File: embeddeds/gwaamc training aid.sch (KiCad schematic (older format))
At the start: 18 parts, among them J1 Conn_Coaxial, U1 LM334Z, U1-LSB MCP4162-502(0-5KΩ), U1-MSBs... MCP4162-104(0-100KΩ), U2 LM334Z, U2-LSB MCP4162-502(0-5KΩ), U2-MSBs... MCP4162-104(0-100KΩ), U3-A AD8244ARMZ, U3-B AD8244ARMZ, U3-C AD8244ARMZ, U3-D AD8244ARMZ, U4 74LV138

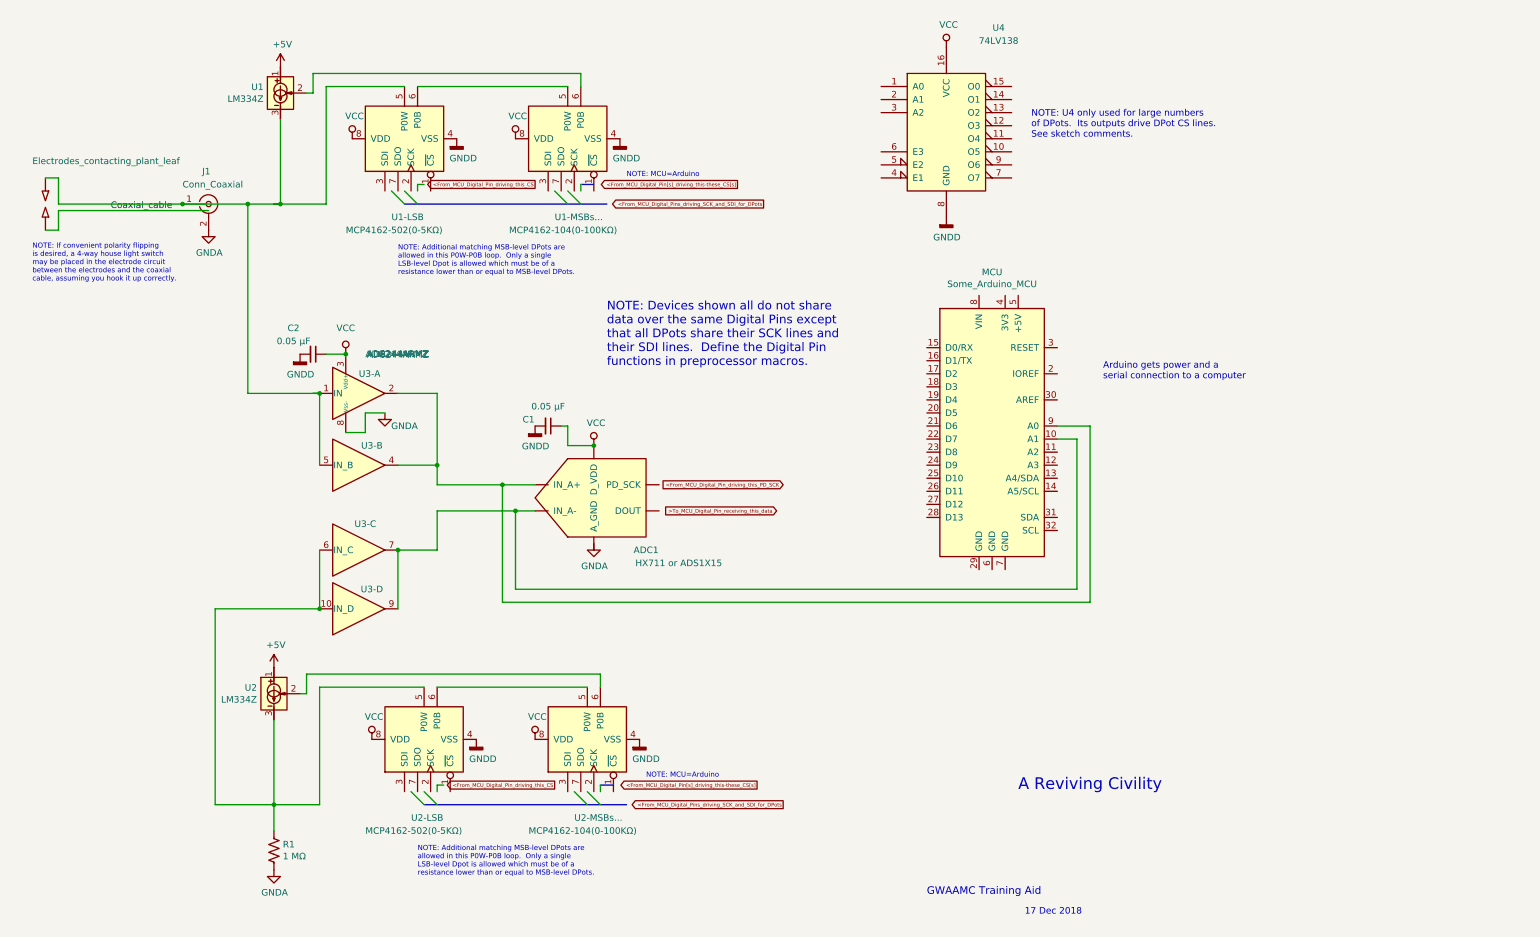
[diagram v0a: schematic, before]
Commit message: Schematic created in KiCad
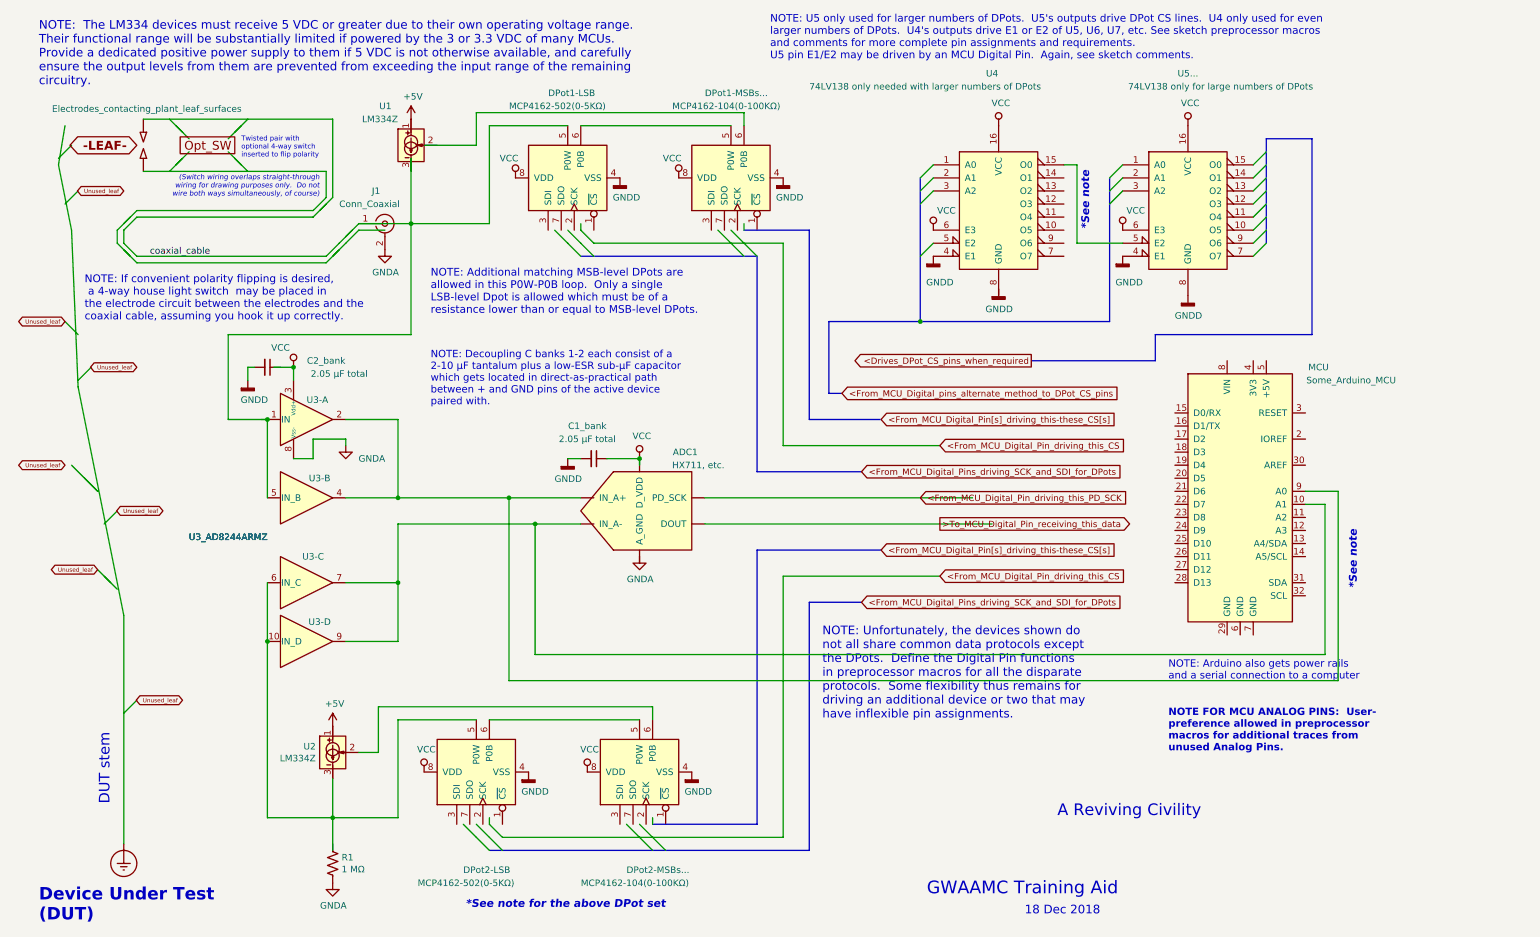
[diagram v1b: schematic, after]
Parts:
- added U4: 74LV138 only needed with larger numbers of DPots, symbol 74xx:74LS138
- ADC1: value HX711 or ADS1X15 -> HX711, etc.
- C1_bank: renamed from C1; value 0.05 µF -> 2.05 µF total
- C2_bank: renamed from C2; value 0.05 µF -> 2.05 µF total
- U3-A: value AD8244ARMZ -> (none)
- U3-B, U3-C, U3-D: value AD8244ARMZ -> U3_AD8244ARMZ
- U5...: renamed from U4; value 74LV138 -> 74LV138 only for large numbers of DPots
- renumbered U1-LSB to DPot1-LSB, U1-MSBs... to DPot1-MSBs..., U2-LSB to DPot2-LSB, U2-MSBs... to DPot2-MSBs..., Electrodes_contacting_plant_leaf to Electrodes_contacting_plant_leaf_surfaces
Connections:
- net labels added: -LEAF-, <Drives_DPot_CS_pins_when_required, <From_MCU_Digital_pins_alternate_method_to_DPot_CS_pins, Earth_Protective, Opt_SW, Unused_leaf, coaxial_cable
- net labels removed: Coaxial_cable
- wire segments 68 -> 90
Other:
- note added: "(Switch wiring overlaps straight-through \nwiring for drawing purposes only. Do not \nwire both ways simultaneously, of course)"
- note added: "*See note"
- note added: "*See note for the above DPot set"
- note added: "18 Dec 2018"
- note added: "DUT stem"
- note added: "Device Under Test \n(DUT)"
- note added: "NOTE FOR MCU ANALOG PINS: User-\npreference allowed in preprocessor \nmacros for additional traces from \nunused Analog Pins."
- note added: "NOTE: Arduino also gets power rails \nand a serial connection to a computer"
- note added: "NOTE: Decoupling C banks 1-2 each consist of a \n2-10 µF tantalum plus a low-ESR sub-µF capacitor \nwhich gets located in direct-as-practical path \nbetween + and GND pins of the active device \npaired with."
- note added: "NOTE: If convenient polarity flipping is desired,\n a 4-way house light switch may be placed in \nthe electrode circuit between the electrodes and the \ncoaxial cable, assuming you hook it up correctly."
- note added: "NOTE: The LM334 devices must receive 5 VDC or greater due to their own operating voltage range. \nTheir functional range will be substantially limited if powered by the 3 or 3.3 VDC of many MCUs. \nProvide a dedicated positive power supply to them if 5 VDC is not otherwise available, and carefully \nensure the output levels from them are prevented from exceeding the input range of the remaining \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"
- note added: "NOTE: U5 only used for larger numbers of DPots. U5's outputs drive DPot CS lines. U4 only used for even \nlarger numbers of DPots. U4's outputs drive E1 or E2 of U5, U6, U7, etc. See sketch preprocessor macros \nand comments for more complete pin assignments and requirements.\nU5 pin E1/E2 may be driven by an MCU Digital Pin. Again, see sketch comments."
- note added: "NOTE: Unfortunately, the devices shown do \nnot all share common data protocols except \nthe DPots. Define the Digital Pin functions \nin preprocessor macros for all the disparate\nprotocols. Some flexibility thus remains for \ndriving an additional device or two that may \nhave inflexible pin assignments."
- note added: "Twisted pair with \noptional 4-way switch \ninserted to flip polarity"
- note removed: "17 Dec 2018"
- note removed: "Arduino gets power and a \nserial connection to a computer"
- note removed: "NOTE: Devices shown all do not share \ndata over the same Digital Pins except\nthat all DPots share their SCK lines and\ntheir SDI lines. Define the Digital Pin \nfunctions in preprocessor macros."
- note removed: "NOTE: If convenient polarity flipping\nis desired, a 4-way house light switch \nmay be placed in the electrode circuit\nbetween the electrodes and the coaxial\ncable, assuming you hook it up correctly."
- note removed: "NOTE: MCU=Arduino"
- note removed: "NOTE: U4 only used for large numbers \nof DPots. Its outputs drive DPot CS lines.\nSee sketch comments."
- moved on the sheet: ADC1, C1_bank, C2_bank, DPot1-LSB, DPot1-MSBs..., DPot2-LSB, DPot2-MSBs..., Electrodes_contacting_plant_leaf_surfaces, J1, MCU, R1, U1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

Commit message: Add files via upload
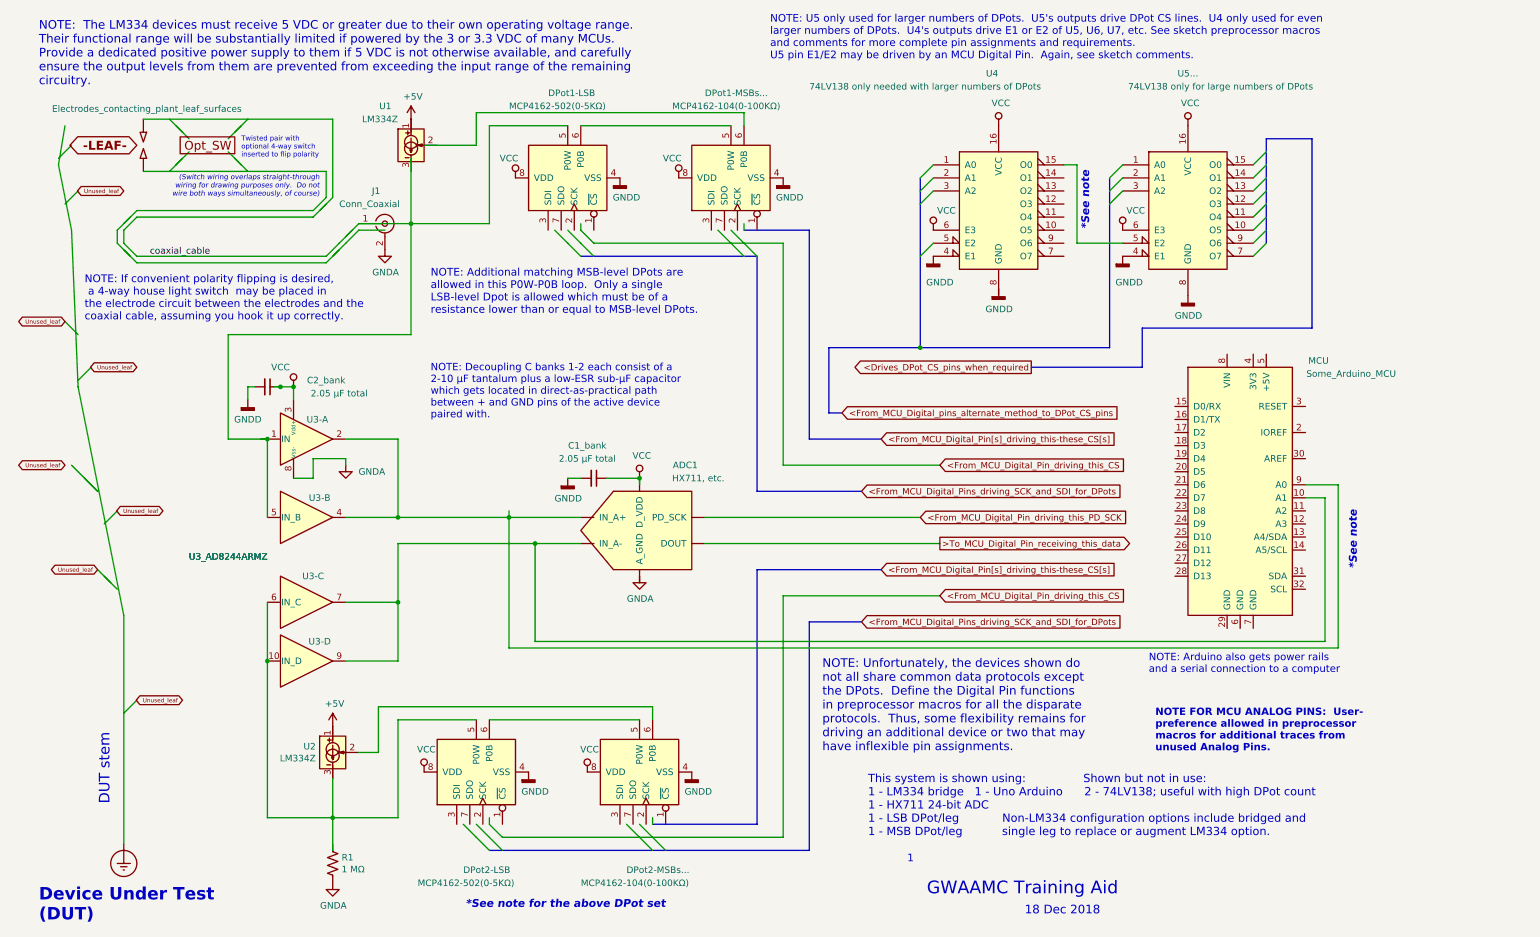
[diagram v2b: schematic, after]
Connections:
- wire segments 90 -> 92
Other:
- note added: "1"
- note added: "NOTE: Unfortunately, the devices shown do \nnot all share common data protocols except \nthe DPots. Define the Digital Pin functions \nin preprocessor macros for all the disparate\nprotocols. Thus, some flexibility remains for \ndriving an additional device or two that may \nhave inflexible pin assignments."
- note added: "This system is shown using: Shown but not in use:\n1 - LM334 bridge 1 - Uno Arduino 2 - 74LV138; useful with high DPot count\n1 - HX711 24-bit ADC\n1 - LSB DPot/leg Non-LM334 configuration options include bridged and\n1 - MSB DPot/leg single leg to replace or augment LM334 option."
- note removed: "A Reviving Civility"
- note removed: "NOTE: Unfortunately, the devices shown do \nnot all share common data protocols except \nthe DPots. Define the Digital Pin functions \nin preprocessor macros for all the disparate\nprotocols. Some flexibility thus remains for \ndriving an additional device or two that may \nhave inflexible pin assignments."
- moved on the sheet: ADC1, C1_bank, C2_bank, MCU, U3-A, U3-B, U3-C, U3-D
